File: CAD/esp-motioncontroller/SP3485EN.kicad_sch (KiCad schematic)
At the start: 54 parts, among them J2 Screw_Terminal_01x10, J3 Screw_Terminal_01x10, J4 Screw_Terminal_01x10, J5 Screw_Terminal_01x03, J6 Screw_Terminal_01x10, J8 Screw_Terminal_01x10, U10 AM26LS31CDR, U11 LTV-817S, U12 LTV-817S, U13 LTV-817S, U14 LTV-817S, U2 AM26LV32EIDR, U4 SP3485EN, U5 AM26LS31CDR, U6 LTV-817S, U7 LTV-817S, U8 LTV-817S, U9 LTV-817S

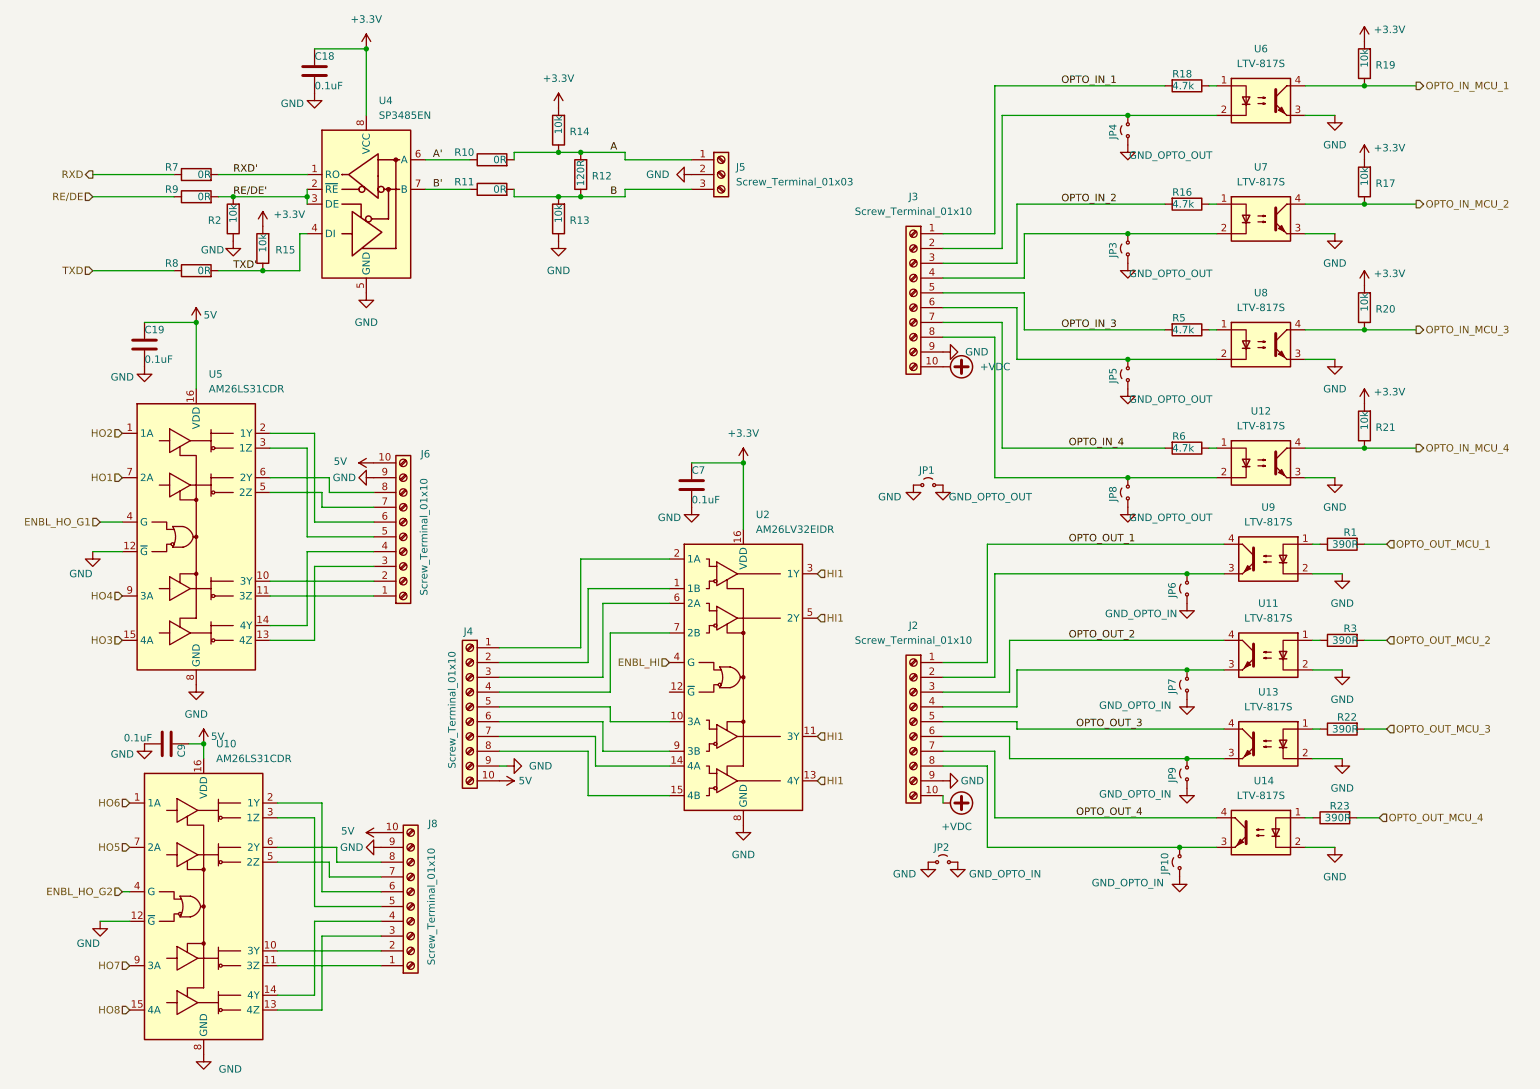
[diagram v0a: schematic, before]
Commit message: Feat: Quaddrivers
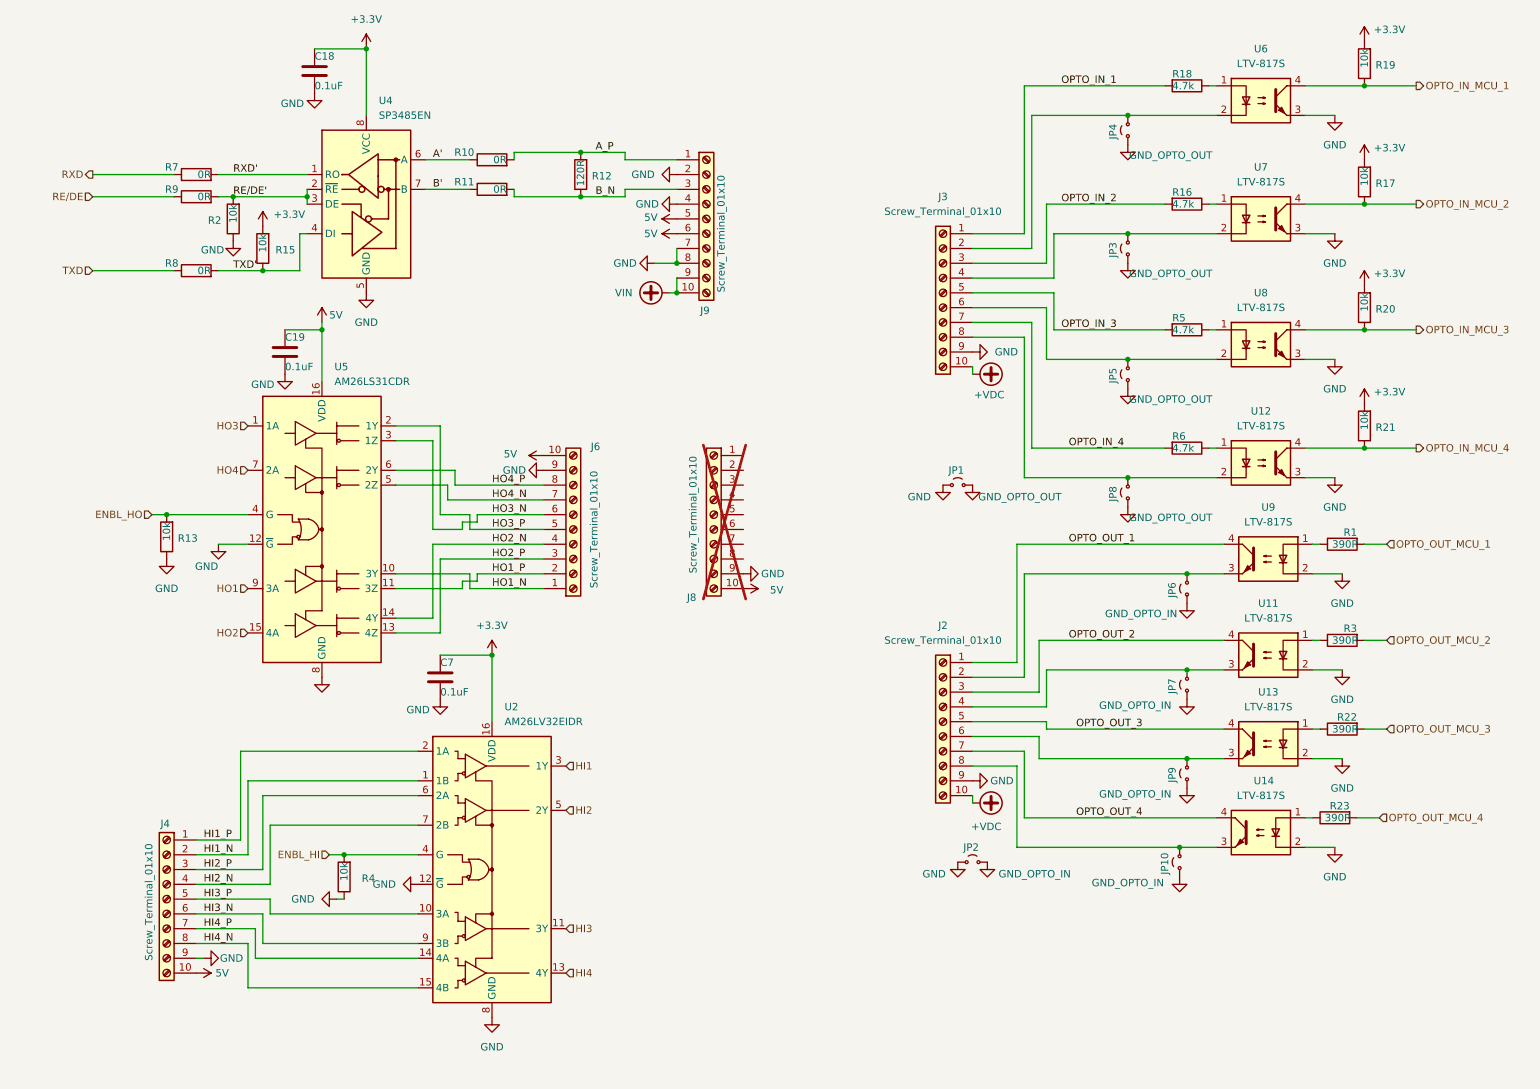
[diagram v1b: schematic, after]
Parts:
- removed C9: 0.1uF, Capacitor_SMD:C_0603_1608Metric, symbol Library:C
- removed J5: Screw_Terminal_01x03, TerminalBlock_Phoenix:TerminalBlock_Phoenix_PT-1,5-3-3.5-H_1x03_P3.50mm_Horizontal, symbol Connector:Screw_Terminal_01x03
- removed R14: 10k, Resistor_SMD:R_0603_1608Metric, symbol Library:R
- removed U10: AM26LS31CDR, Package_SO:SOIC-16_3.9x9.9mm_P1.27mm, symbol Interface:AM26LS31CD
- added J9: Screw_Terminal_01x10, TerminalBlock_Phoenix:TerminalBlock_Phoenix_PT-1,5-10-3.5-H_1x10_P3.50mm_Horizontal, symbol Connector:Screw_Terminal_01x10
- added R4: 10k, Resistor_SMD:R_0603_1608Metric, symbol Library:R
- C7: LCSC Part # - -> C14663
- J2, J3, J4, J6: LCSC Part # (none) -> C5184956
- J8: LCSC Part # (none) -> C5184956; now not fitted; now left out of the parts list
- U2: LCSC Part # (none) -> C527448
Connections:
- net 5V: now also J9.5 (Pin_5), J9.6 (Pin_6)
- net ENBL_HI: now also R4.2
- net GND: now also U2.12 (~{G}), J9.2 (Pin_2), J9.4 (Pin_4), J9.7 (Pin_7), J9.8 (Pin_8), R4.1
- net HI1: no longer U2.11 (3Y), U2.13 (4Y), U2.5 (2Y)
- net HO1: now also U5.9 (3A); no longer U5.7 (2A)
- net HO2: now also U5.15 (4A); no longer U5.1 (1A)
- net HO3: now also U5.1 (1A); no longer U5.15 (4A)
- net HO4: now also U5.7 (2A); no longer U5.9 (3A)
- net HO1_N: now reaches J6.1 (Pin_1)
- net HO1_N: now also U5.10 (3Y); no longer U5.11 (3Z)
- net HO1_P: now reaches J6.2 (Pin_2)
- net HO1_P: now also U5.11 (3Z); no longer U5.10 (3Y)
- net HO2_P: now reaches J6.3 (Pin_3), U5.13 (4Z)
- net HO2_N: now reaches J6.4 (Pin_4), U5.14 (4Y)
- net HO3_N: now reaches U5.3 (1Z)
- net HO3_N: now also J6.6 (Pin_6); no longer J6.5 (Pin_5)
- net HO3_P: now reaches U5.2 (1Y)
- net HO3_P: now also J6.5 (Pin_5); no longer J6.6 (Pin_6)
- net HO4_N: now reaches J6.7 (Pin_7), U5.5 (2Z)
- net HO4_P: now reaches J6.8 (Pin_8), U5.6 (2Y)
- net HI1_P: now reaches J4.1 (Pin_1), U2.2 (1A)
- net HI1_N: now reaches J4.2 (Pin_2), U2.1 (1B)
- net HI2_P: now reaches J4.3 (Pin_3), U2.6 (2A)
- net HI2_N: now reaches J4.4 (Pin_4), U2.7 (2B)
- net HI3_P: now reaches J4.5 (Pin_5), U2.10 (3A)
- net HI3_N: now reaches J4.6 (Pin_6), U2.9 (3B)
- net HI4_P: now reaches J4.7 (Pin_7), U2.14 (4A)
- net HI4_N: now reaches J4.8 (Pin_8), U2.15 (4B)
- net A renamed A_P
- net A_P: now also J9.1 (Pin_1)
- net B renamed B_N
- net B_N: now also J9.3 (Pin_3); no longer R13.2
- net ENBL_HO_G1 renamed ENBL_HO
- net ENBL_HO: now also R13.2
- new net HI2: U2.5 (2Y)
- new net HI3: U2.11 (3Y)
- new net HI4: U2.13 (4Y)
- new net VIN: J9.10 (Pin_10), J9.9 (Pin_9)
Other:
- moved on the sheet: C19, C7, J2, J3, J4, J6, JP1, JP2, U2, U5
